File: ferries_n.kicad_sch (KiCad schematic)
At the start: 47 parts

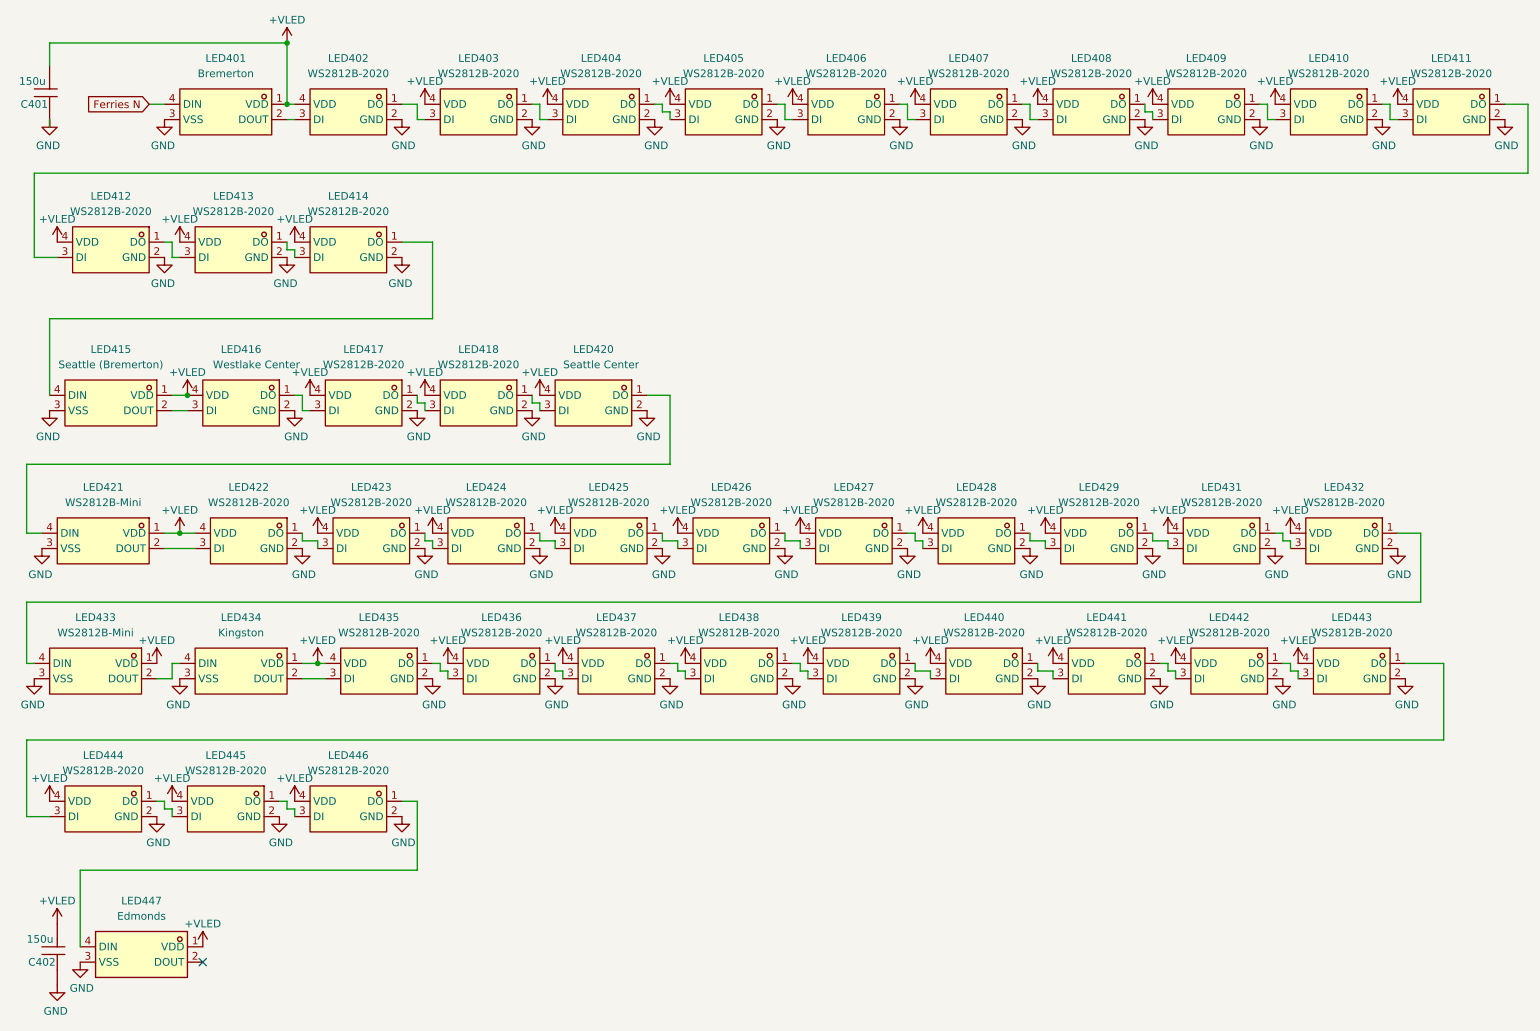
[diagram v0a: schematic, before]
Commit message: sounder layout checkpoint
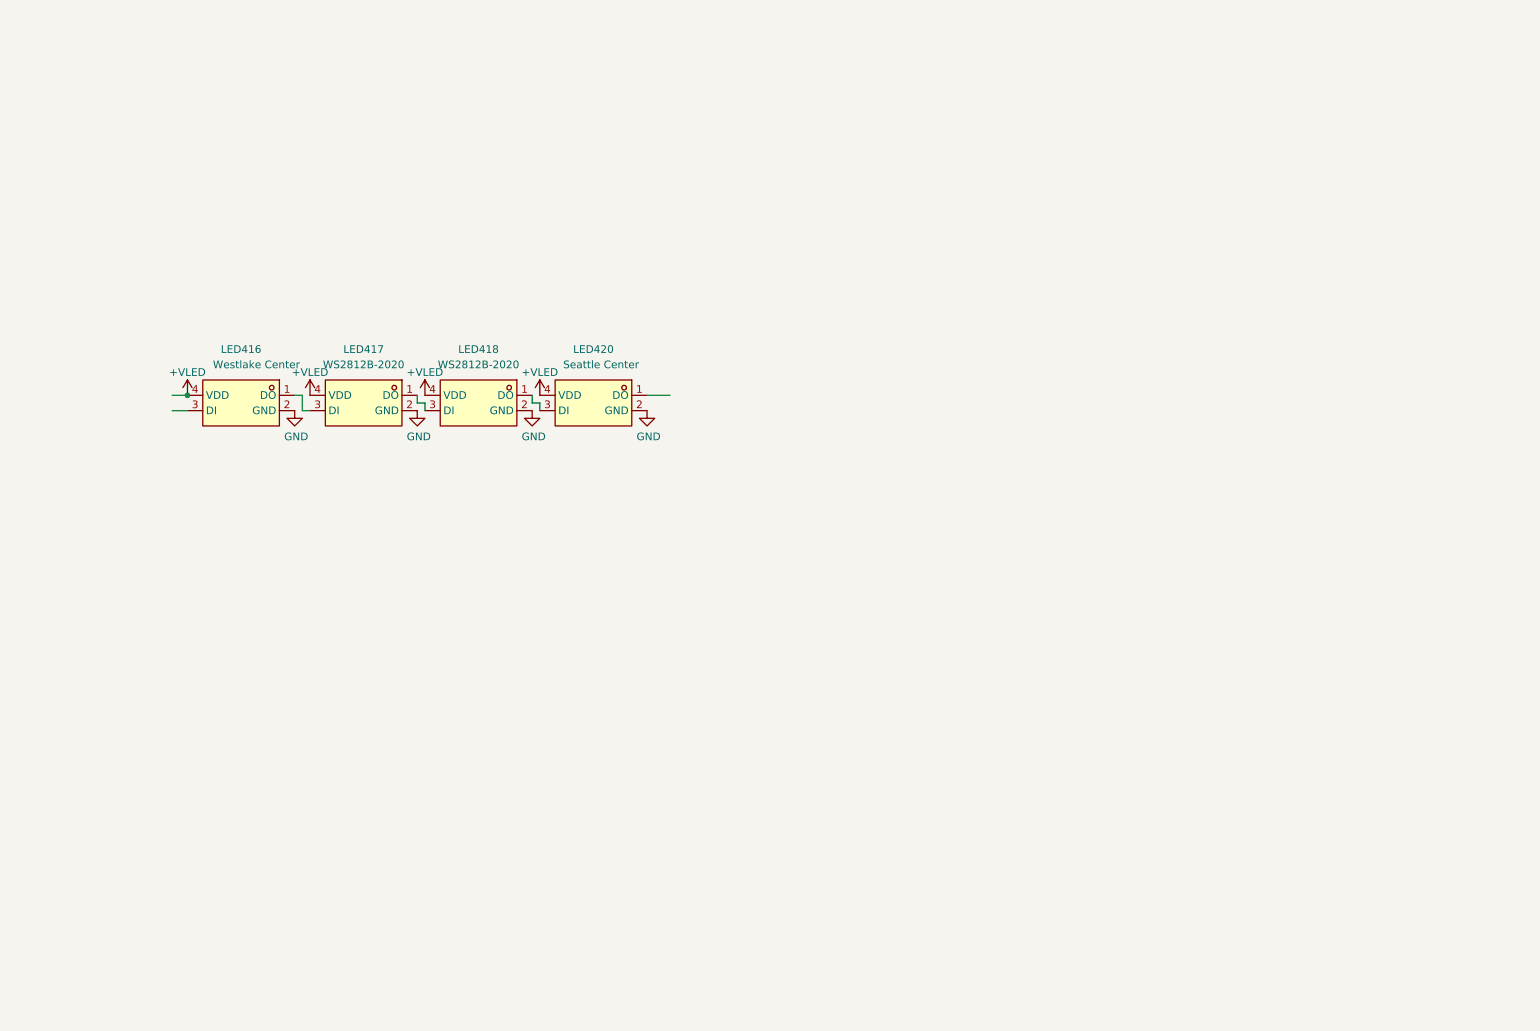
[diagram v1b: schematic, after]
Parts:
- removed C401, C402: 150u, EasyEDA:CAP-SMD_L3.5-W2.8, symbol EasyEDA:CL21B106KOQNNNE
- removed LED401, LED415, LED421, LED433, LED434, LED447: WS2812B-Mini, EasyEDA:LED-SMD_4P-L3.5-W3.5-TL_WS2812B, symbol EasyEDA:WS2812B-MINI
- removed LED402, LED403, LED404, LED405, LED406, LED407, LED408, LED409, LED410, LED411, LED412, LED413, LED414, LED422, LED423, LED424, LED425, LED426, LED427, LED428, LED429, LED431, LED432, LED435, LED436, LED437, LED438, LED439, LED440, LED441, LED442, LED443, LED444, LED445, LED446: WS2812B-2020, EasyEDA:LED-SMD_4P-L2.0-W2.0-TL_WS2812B-2020, symbol EasyEDA:WS2812B-2020
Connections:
- no-connect marks 1 -> 0
